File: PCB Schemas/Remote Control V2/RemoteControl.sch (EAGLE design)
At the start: 23 parts, among them IC1 ATMEGA328-PU, Q1 16MHz

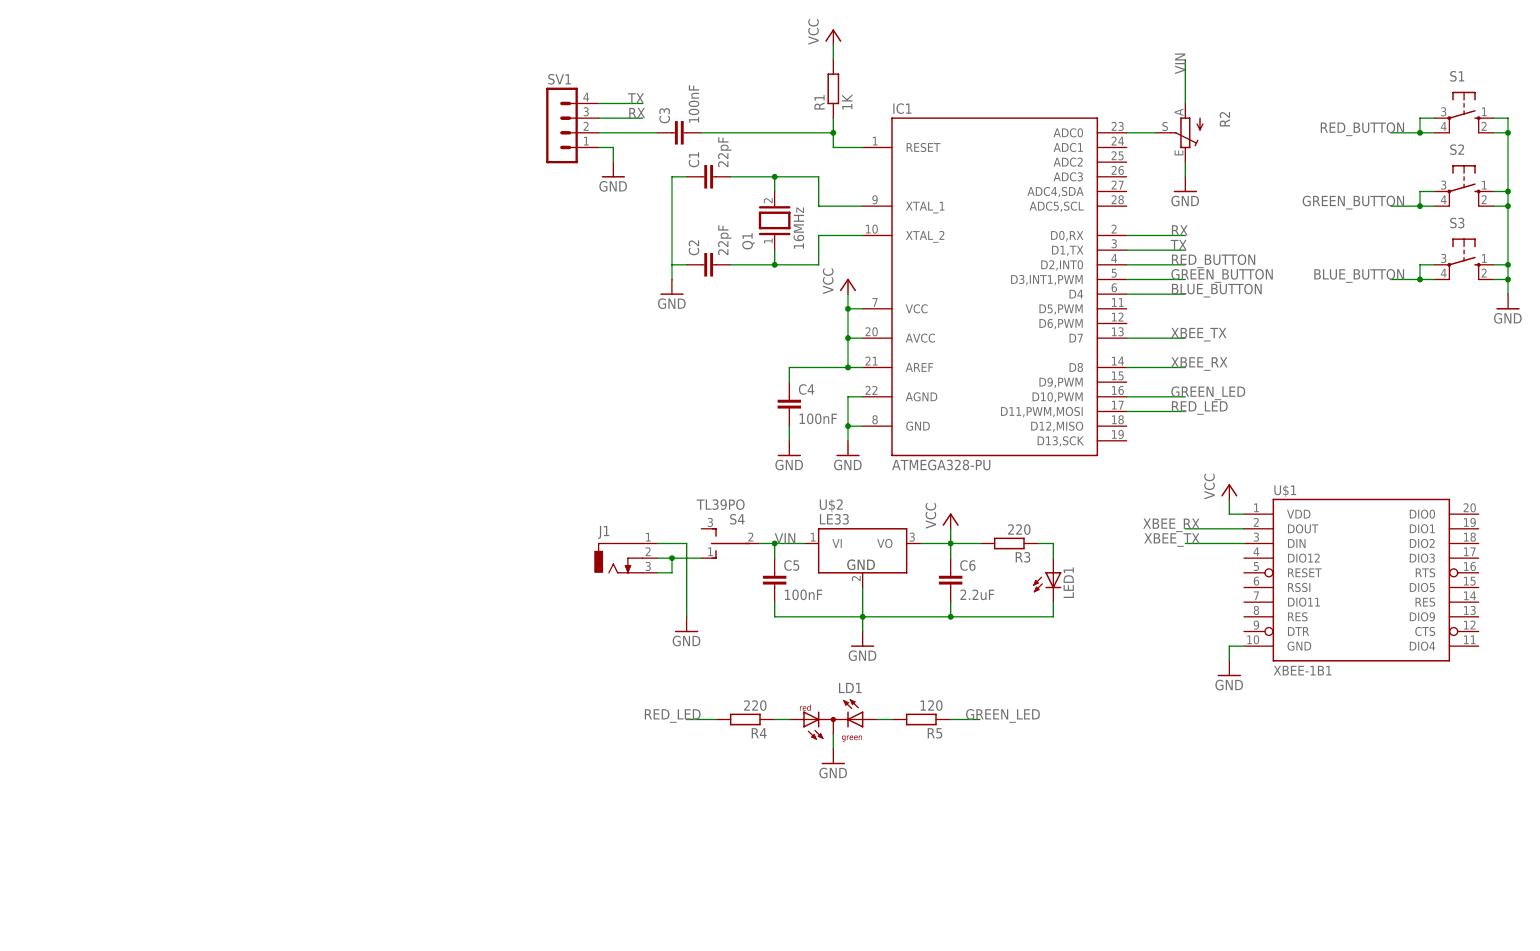
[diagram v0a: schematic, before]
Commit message: Finalized V1 and V2 of remote control
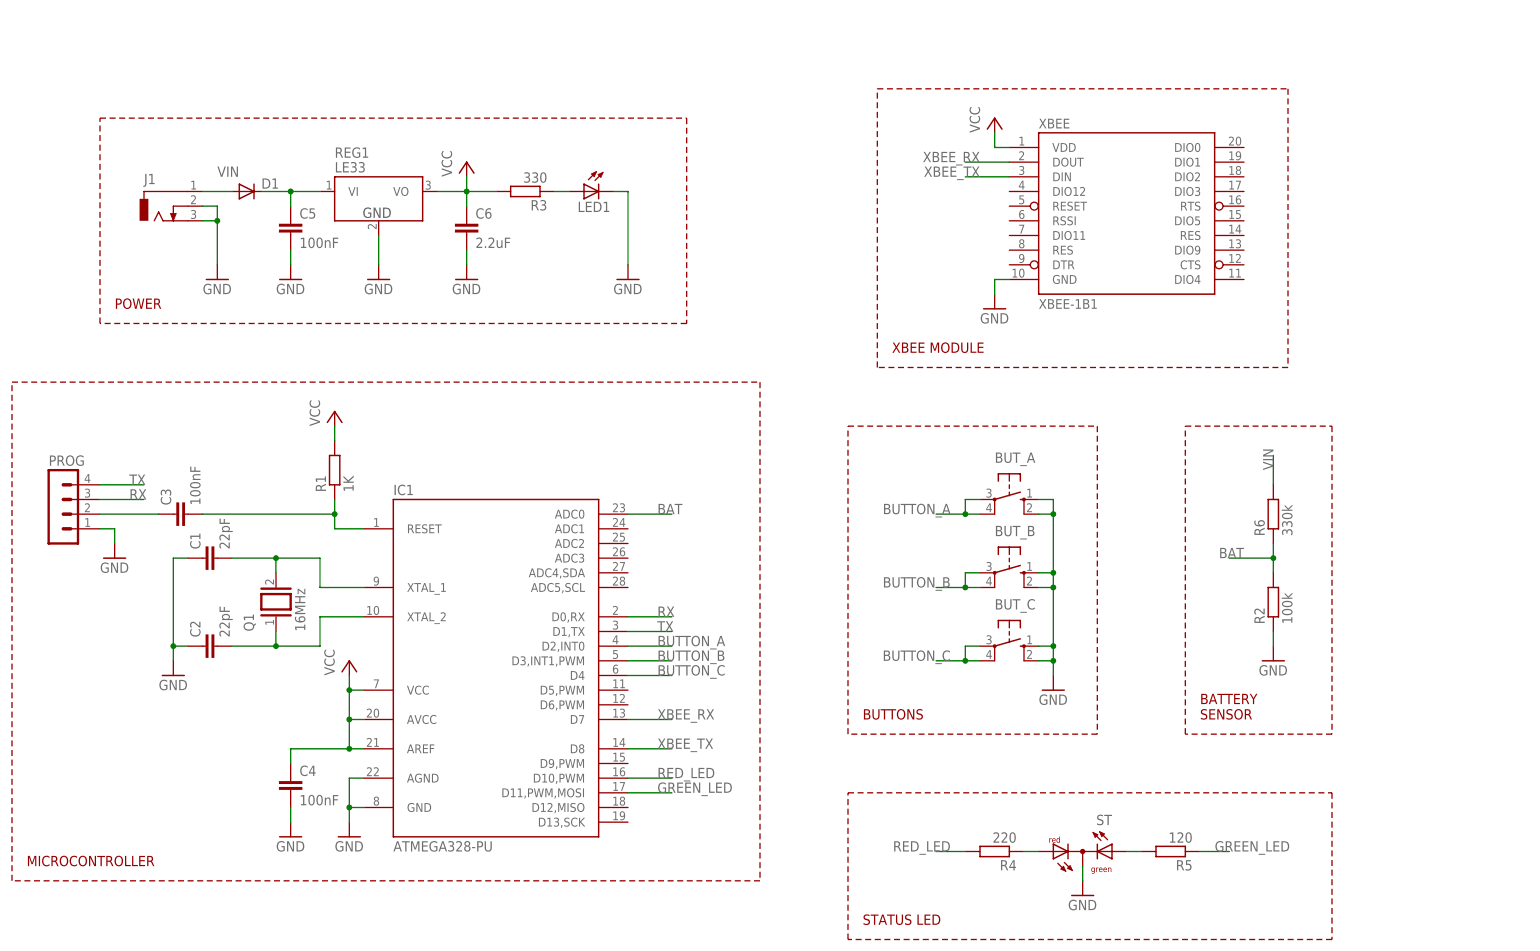
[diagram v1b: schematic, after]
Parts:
- removed LD1: (no value), led:DUOLED-RG-C
- removed S1, S2, S3: (no value), switch-omron:40-XX
- removed S4: TL39PO, switch:TL39PO
- removed SV1: (no value), con-lstb:MA04-1
- removed U$1: XBEE-1B1, Xbee:XBEE-1B1
- removed U$2: LE33, Regulator:LE33
- added BUT_A, BUT_B, BUT_C: (no value), switch-omron:40-XX
- added D1: 1N4148DO35-7, diode:1N4148DO35-7
- added PROG: (no value), con-lstb:MA04-1
- added R6: 330k, resistor:R-EU_0207/7
- added REG1: LE33, Regulator:LE33
- added ST: (no value), led:DUOLED-RG-C
- added XBEE: XBEE-1B1, Xbee:XBEE-1B1
- J1: device con-jack:DCJ0303 -> Connectors:DCJ0303
- R2: value (none) -> 100k; device pot:TRIM_EU-CA9V -> resistor:R-EU_0207/7
- R3: value 220 -> 330
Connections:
- removed net BLUE_BUTTON: IC1.D4, S3.P, S3.P1
- removed net GREEN_BUTTON: IC1.D3,INT1,PWM, S2.P, S2.P1
- removed net N$9: IC1.ADC0, R2.S
- removed net RED_BUTTON: IC1.D2,INT0, S1.P, S1.P1
- new net BAT: IC1.ADC0, R2.2, R6.1
- new net BUTTON_A: BUT_A.P, BUT_A.P1, IC1.D2,INT0
- new net BUTTON_B: BUT_B.P, BUT_B.P1, IC1.D3,INT1,PWM
- new net BUTTON_C: BUT_C.P, BUT_C.P1, IC1.D4
- net GND: now also BUT_A.S, BUT_A.S1, BUT_B.S, BUT_B.S1, BUT_C.S, BUT_C.S1, J1.2, J1.3, PROG.1, R2.1, REG1.GND, ST.C, XBEE.GND; no longer J1.1, LD1.C, R2.E, S1.S, S1.S1, S2.S, S2.S1, S3.S, S3.S1, SV1.1, U$1.GND, U$2.GND
- net GREEN_LED: now also IC1.D11,PWM,MOSI; no longer IC1.D10,PWM
- net N$11: now also ST.AR; no longer LD1.AR
- net N$12: now also ST.AG; no longer LD1.AG
- net N$3: now also C5.1, D1.C, REG1.VI; no longer J1.2, J1.3, S4.O
- net N$6: now also PROG.2; no longer SV1.2
- net RED_LED: now also IC1.D10,PWM; no longer IC1.D11,PWM,MOSI
- net RX: now also PROG.3; no longer SV1.3
- net TX: now also PROG.4; no longer SV1.4
- net VCC: now also REG1.VO, XBEE.VDD; no longer U$1.VDD, U$2.VO
- net VIN: now also D1.A, J1.1, R6.2; no longer C5.1, R2.A, S4.P, U$2.VI
- net XBEE_RX: now also IC1.D7, XBEE.DOUT; no longer IC1.D8, U$1.DOUT
- net XBEE_TX: now also IC1.D8, XBEE.DIN; no longer IC1.D7, U$1.DIN
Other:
- note added: "BATTERY SENSOR"
- note added: "BUTTONS"
- note added: "MICROCONTROLLER"
- note added: "POWER"
- note added: "STATUS LED"
- note added: "XBEE MODULE"
- moved on the sheet: C1, C2, C3, C4, C5, C6, IC1, J1, LED1, Q1, R1, R3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
